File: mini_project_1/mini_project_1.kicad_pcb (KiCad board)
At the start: 2 copper layers, 26.4 x 14.3 mm, 17 parts, among them J1 480370001, U2 MCP1700x-330xxTT, U3 MCP602

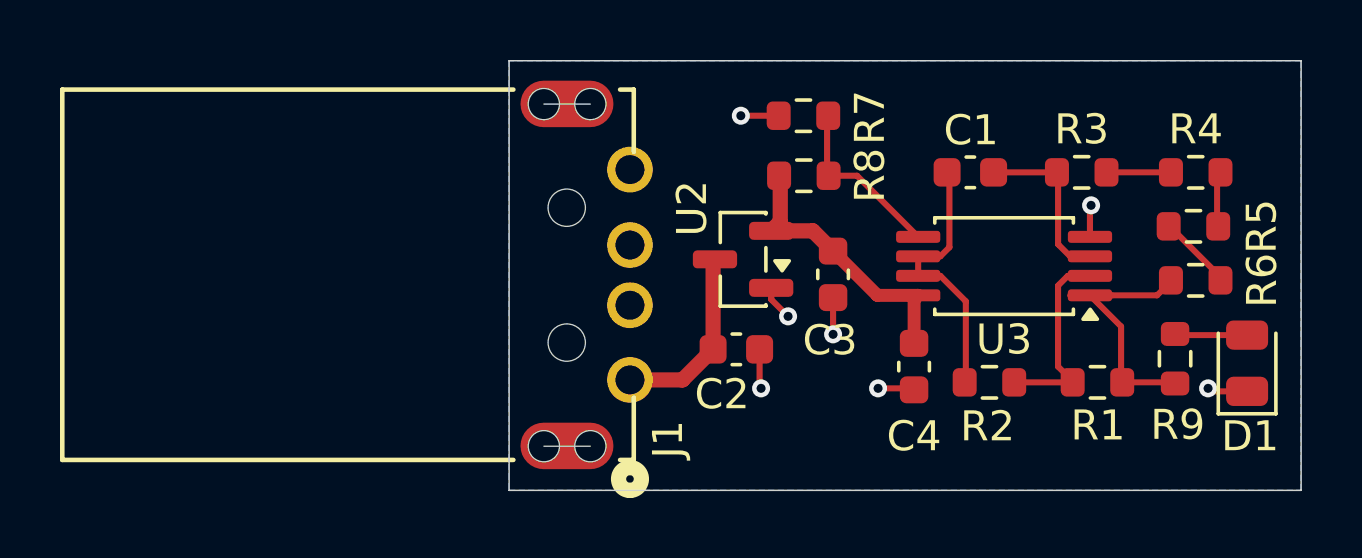
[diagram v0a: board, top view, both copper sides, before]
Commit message: Add complete schematic, layout, report, sim
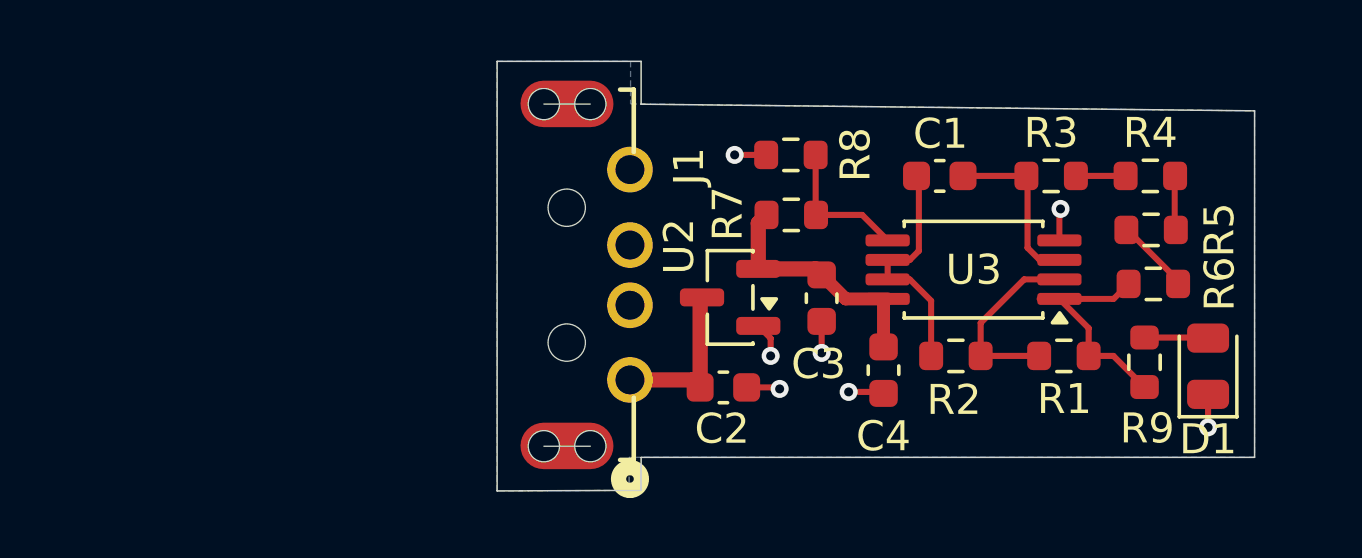
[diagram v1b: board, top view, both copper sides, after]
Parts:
- moved R4 1.52 mm to (156.1, 97.7)
- moved R1 1.42 mm to (153.2, 103.7)
- moved R2 1.42 mm to (149.6, 103.7)
- moved R5 1.42 mm to (156.1, 99.5)
- moved R6 1.42 mm to (156.2, 101.3)
- moved R7 1.37 mm to (144.1, 99.0)
- moved R8 1.37 mm to (144.1, 97.0)
- moved C2 1.34 mm to (141.8, 104.8)
- moved U2 1.34 mm to (142.1, 101.8)
- moved D1 1.30 mm to (158.0, 104.1)
- moved R9 1.03 mm to (155.9, 103.9)
- moved C1 1.03 mm to (149.1, 97.7)
- moved R3 1.03 mm to (152.8, 97.7)
- moved U3 1.03 mm to (150.2, 100.8)
- moved C4 1.03 mm to (147.2, 104.2)
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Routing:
- net +3.3V: track 9.31 -> 8.00 mm
- net Net-(U3B-+): track 5.89 -> 4.74 mm
- net /+1.65: track 8.98 -> 7.93 mm
- net GND: track 8.87 -> 7.85 mm
- net Net-(R1-Pad2): track 9.47 -> 8.51 mm
- net Net-(J1-VBUS): track 6.22 -> 5.47 mm
- net Net-(R3-Pad2): track 2.23 -> 1.66 mm
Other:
- board size 26.4 x 14.3 mm -> 25.2 x 14.3 mm
